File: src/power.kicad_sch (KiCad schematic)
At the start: 51 parts, among them CN8 POWER, U10B1 74LS244, U11B1 74LS373, U12B1 74LS244, U13B1 74LS373, U1B1 68000D, U2B1 FAT_AGNUS_8375, U32C1 74LS139, U34B1 74LS373, U35B1 74LS244, U36G1 74LS05, U37E1 74LS32, U5C1 GARY_5719, X1B1 XTAL

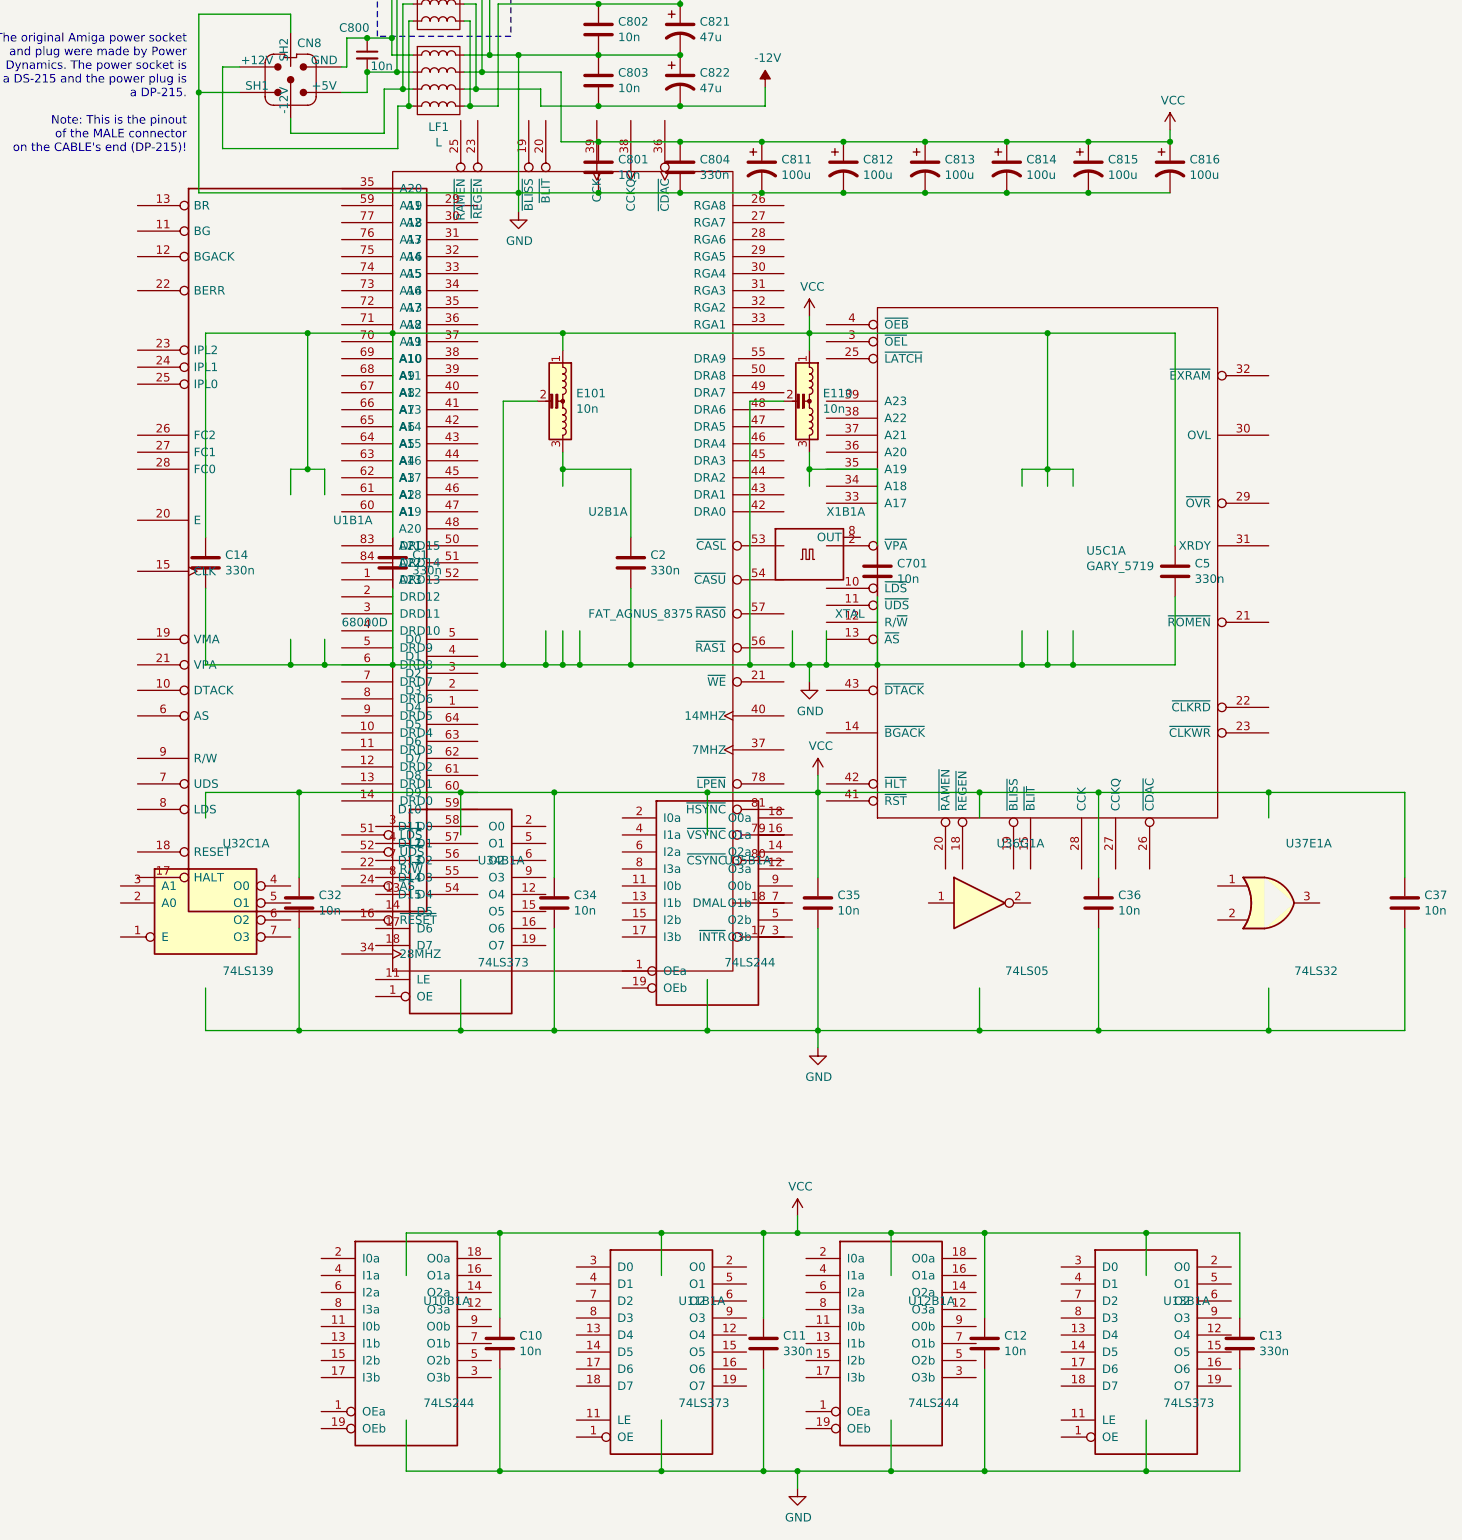
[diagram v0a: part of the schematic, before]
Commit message: kicad 10
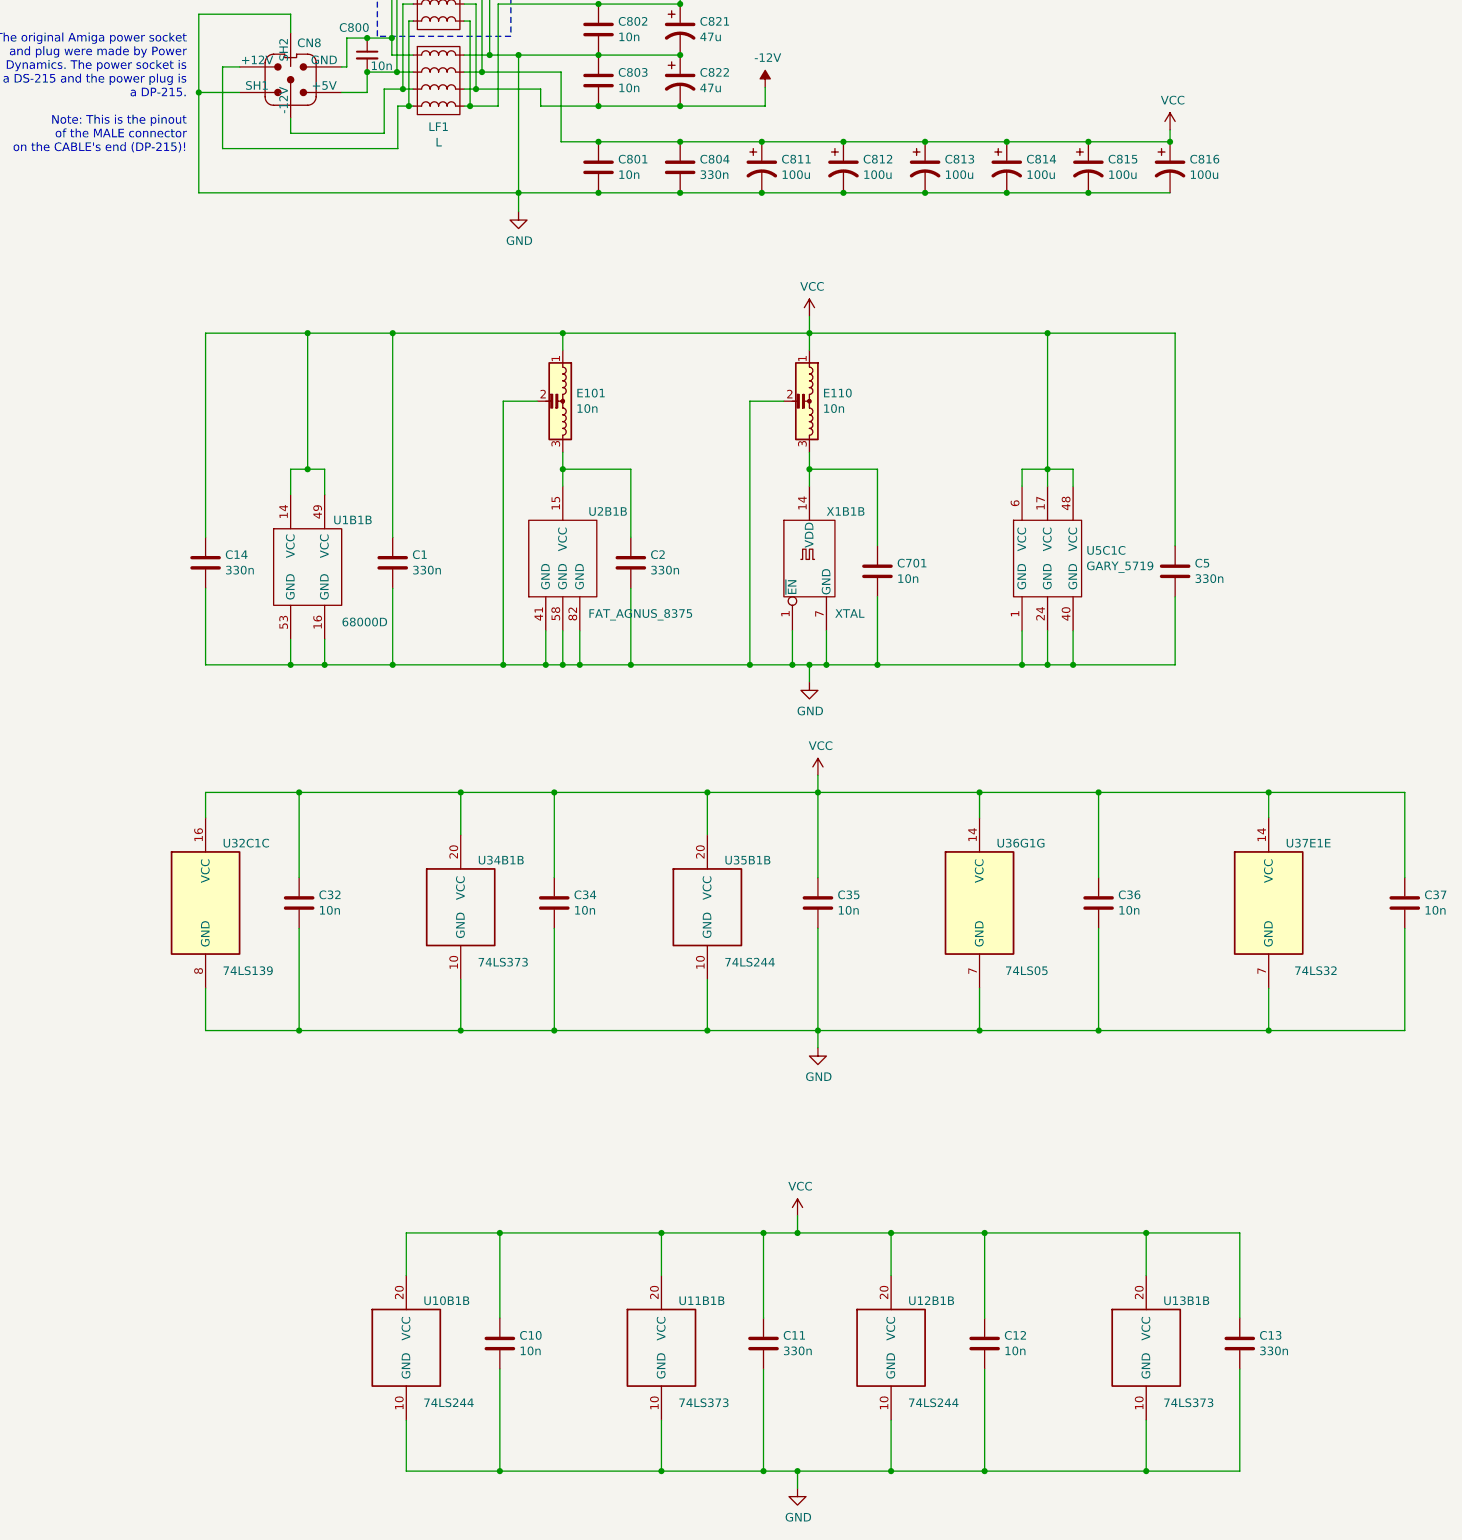
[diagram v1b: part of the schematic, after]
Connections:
- net GND: now also U10B1.10 (GND), U11B1.10 (GND), U12B1.10 (GND), U13B1.10 (GND), U1B1.16 (GND), U1B1.53 (GND), U2B1.41 (GND), U2B1.58 (GND), U2B1.82 (GND), U32C1.8 (GND), U34B1.10 (GND), U35B1.10 (GND), U36G1.7 (GND), U37E1.7 (GND), U5C1.1 (GND), U5C1.24 (GND), U5C1.40 (GND), X1B1.1 (~{EN}), X1B1.7 (GND)
- net VCC: now also U10B1.20 (VCC), U11B1.20 (VCC), U12B1.20 (VCC), U13B1.20 (VCC), U1B1.14 (VCC), U1B1.49 (VCC), U32C1.16 (VCC), U34B1.20 (VCC), U35B1.20 (VCC), U36G1.14 (VCC), U37E1.14 (VCC), U5C1.17 (VCC), U5C1.48 (VCC), U5C1.6 (VCC)
- net at C2.1, E101.3: now also U2B1.15 (VCC)
- net at C701.1, E110.3: now also X1B1.14 (VDD)
